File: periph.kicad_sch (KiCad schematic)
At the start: 20 parts, among them Q1 Q_NMOS_GSD, U13 MQ-6, U14 BME680, U15 LSM6DS3

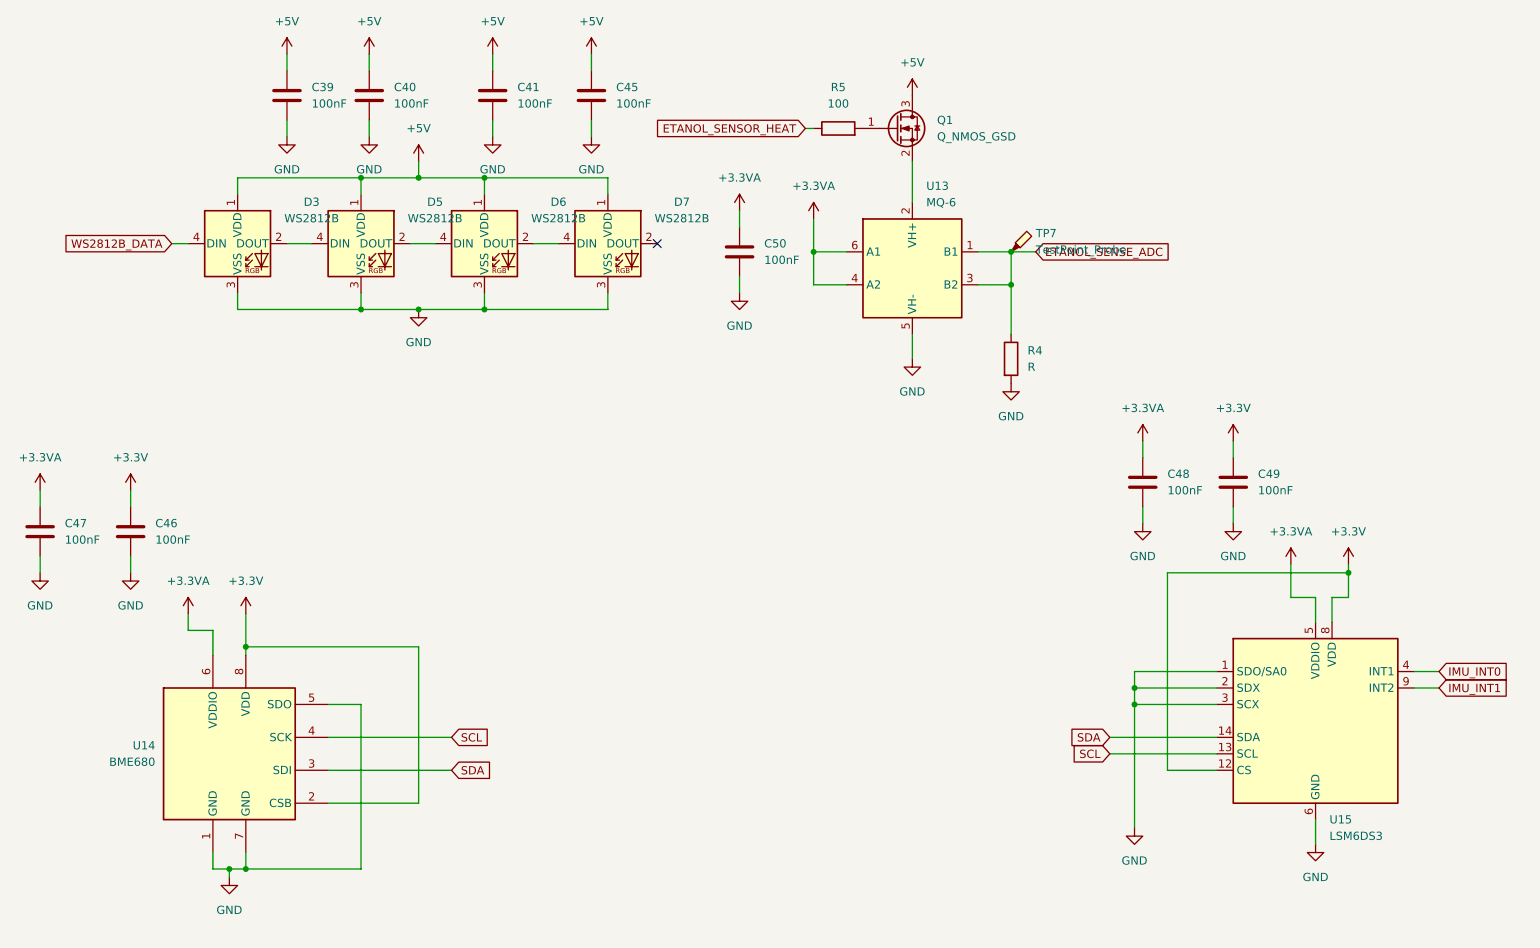
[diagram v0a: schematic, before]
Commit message: Do compoent placing
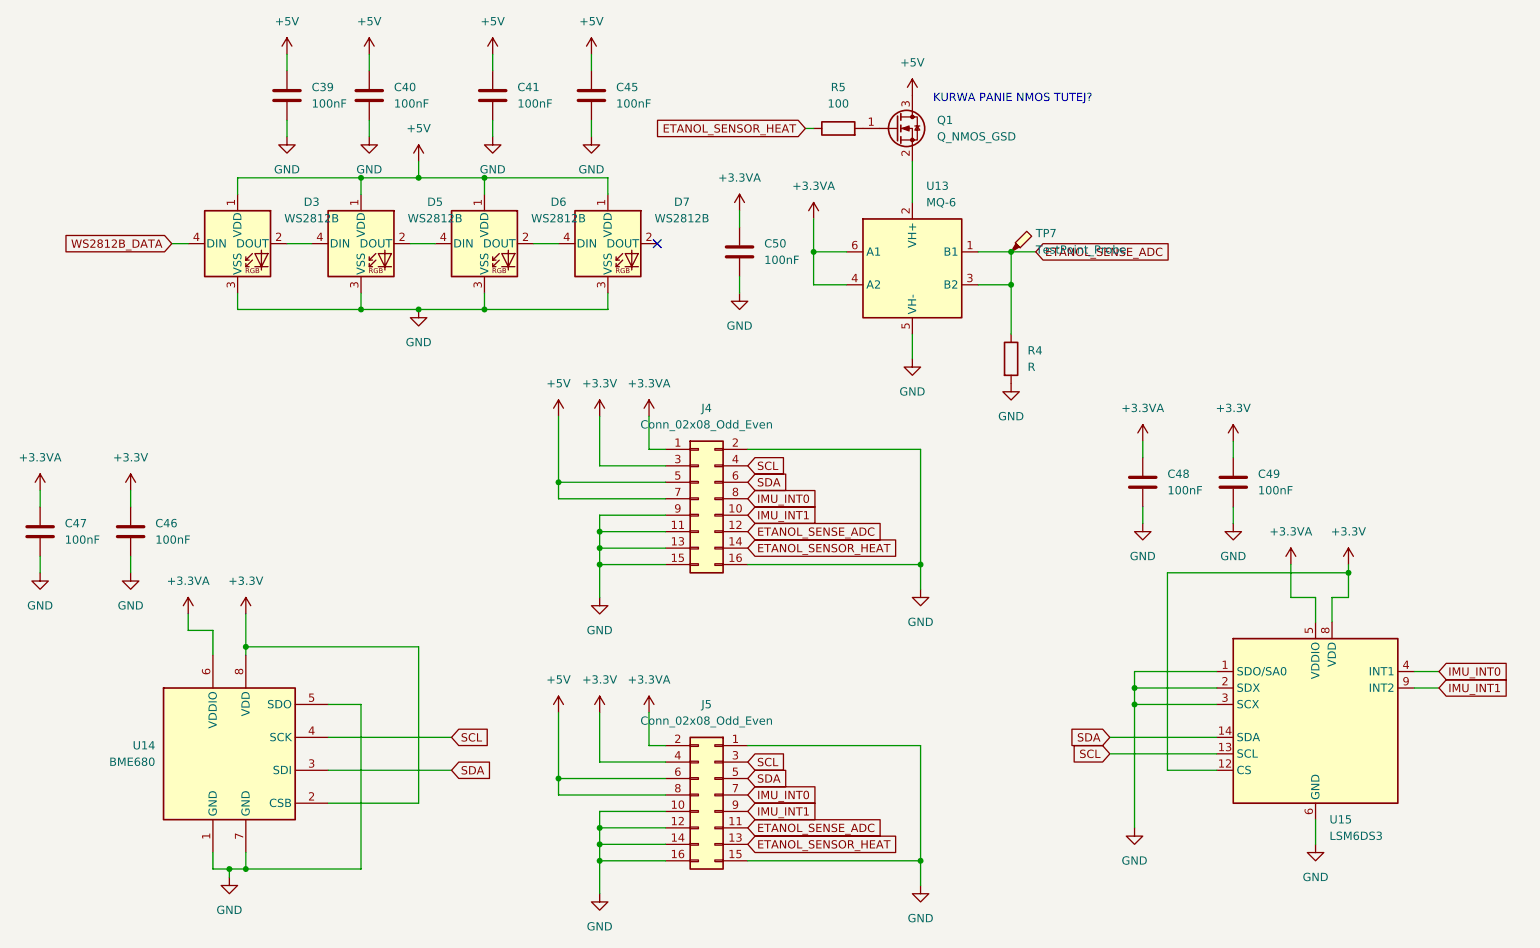
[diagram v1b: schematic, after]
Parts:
- added J4, J5: Conn_02x08_Odd_Even, Connector_PinHeader_2.54mm:PinHeader_2x08_P2.54mm_Vertical, symbol Connector_Generic:Conn_02x08_Odd_Even
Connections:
- net +3.3V: now also J4.3 (Pin_3), J5.4 (Pin_4)
- net +3.3VA: now also J4.1 (Pin_1), J5.2 (Pin_2)
- net +5V: now also J4.5 (Pin_5), J4.7 (Pin_7), J5.6 (Pin_6), J5.8 (Pin_8)
- net ETANOL_SENSE_ADC: now also J4.12 (Pin_12), J5.11 (Pin_11)
- net ETANOL_SENSOR_HEAT: now also J4.14 (Pin_14), J5.13 (Pin_13)
- net GND: now also J4.11 (Pin_11), J4.13 (Pin_13), J4.15 (Pin_15), J4.16 (Pin_16), J4.2 (Pin_2), J4.9 (Pin_9), J5.1 (Pin_1), J5.10 (Pin_10), J5.12 (Pin_12), J5.14 (Pin_14), J5.15 (Pin_15), J5.16 (Pin_16)
- net IMU_INT0: now also J4.8 (Pin_8), J5.7 (Pin_7)
- net IMU_INT1: now also J4.10 (Pin_10), J5.9 (Pin_9)
- net SCL: now also J4.4 (Pin_4), J5.3 (Pin_3)
- net SDA: now also J4.6 (Pin_6), J5.5 (Pin_5)
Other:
- note added: "KURWA PANIE NMOS TUTEJ?"
